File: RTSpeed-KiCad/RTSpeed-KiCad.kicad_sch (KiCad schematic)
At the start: 91 parts, among them J1 24V IN, J2 USB C Receptacle, J3 MOTOR, J4 -, J5 -, J6 -, J7 SWD-I^{2}C, J8 SENSORES HALL, Q1 DMG3402L, SW1 BOOT0, SW2 NRST, U1 STM32F411CEUx, U2 LM317L, U3 ADS7830, U4 LM317, Y1 25MHz, Y2 32.768kHz

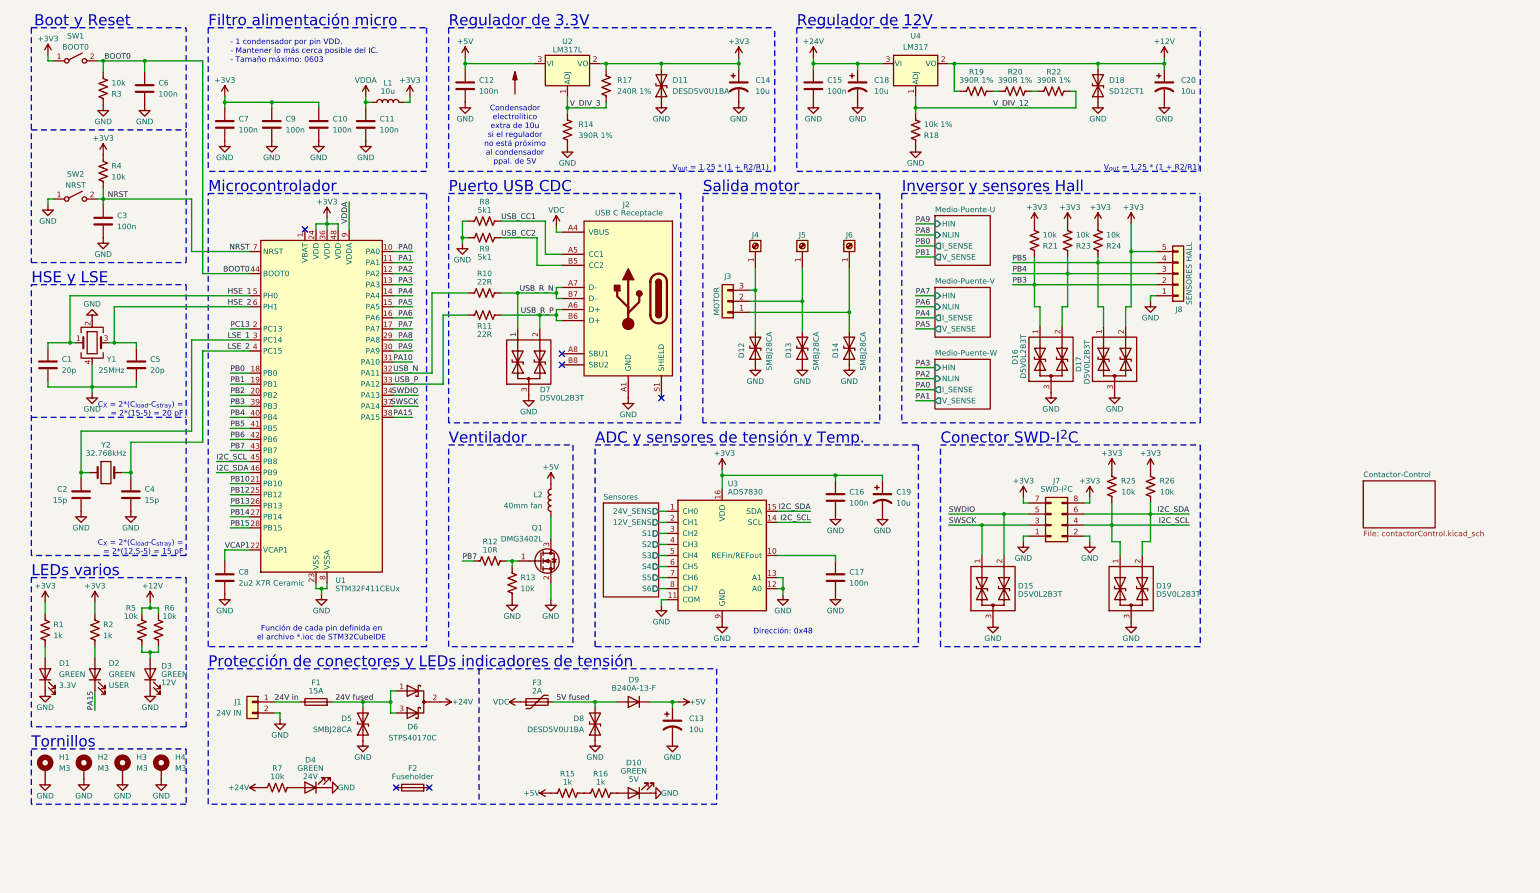
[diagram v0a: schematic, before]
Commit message: PCB redesign (not final)
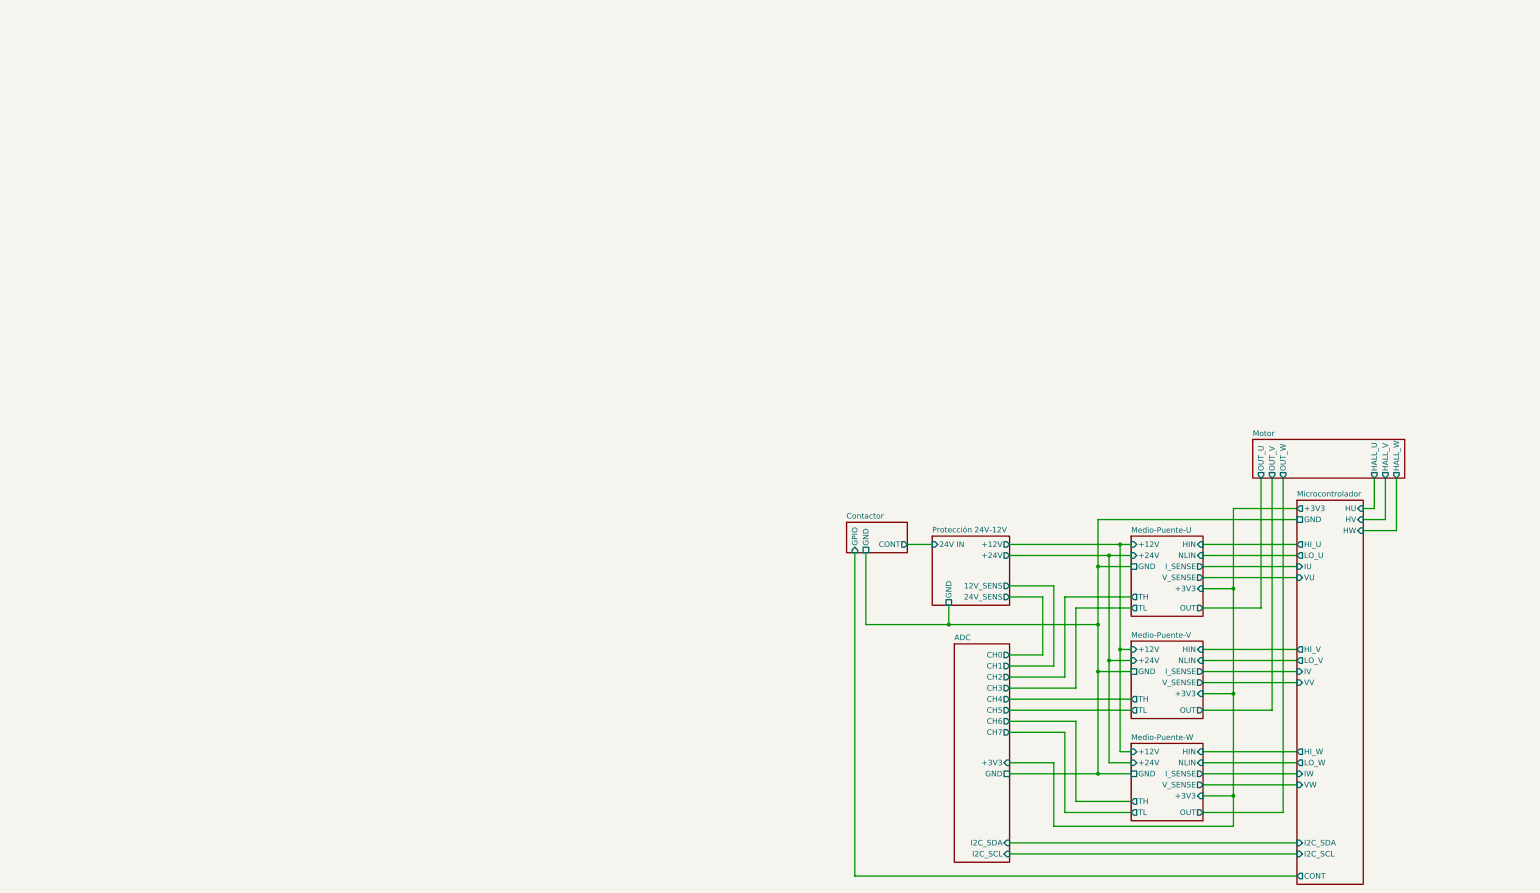
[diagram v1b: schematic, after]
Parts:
- removed C1, C5: 20p, Capacitor_SMD:C_0603_1608Metric, symbol Device:C
- removed C10, C11, C12, C15, C16, C17, C3, C6, C7, C9: 100n, Capacitor_SMD:C_0603_1608Metric, symbol Device:C
- removed C13, C14, C18, C19, C20: 10u, Capacitor_SMD:CP_Elec_4x5.4, symbol Device:C_Polarized_US
- removed C2, C4: 15p, Capacitor_SMD:C_0603_1608Metric, symbol Device:C
- removed C8: 2u2 X7R Ceramic, Capacitor_SMD:C_0603_1608Metric, symbol Device:C
- removed D1, D10, D2, D3, D4: GREEN, LED_SMD:LED_0805_2012Metric, symbol Device:LED
- removed D11, D8: DESD5V0U1BA, Diode_SMD:D_SOD-323_HandSoldering, symbol Device:D_TVS
- removed D12, D13, D14, D5: SMBJ28CA, Diode_SMD:D_SMB, symbol Device:D_TVS
- removed D15, D16, D17, D19, D7: D5V0L2B3T, Package_TO_SOT_SMD:SOT-523, symbol TFG-Brushless-ESC:Dual-TVS
- removed D18: SD12CT1, Diode_SMD:D_SOD-323_HandSoldering, symbol Device:D_TVS
- removed D6: STPS40170C, Package_TO_SOT_THT:TO-220-3_Vertical, symbol Device:D_Schottky_Dual_CommonCathode_AKA_Parallel
- removed D9: B240A-13-F, Diode_SMD:D_SMA, symbol Diode:1N4148W
- removed F1: 15A, TFG-Brushless-ESC:Fuseholder_Automotive, symbol Device:Fuse
- removed F2: Fuseholder, symbol Device:Fuse
- removed F3: 2A, Fuse:Fuse_1812_4532Metric, symbol Device:Polyfuse
- removed H1, H2, H3, H4: M3, MountingHole:MountingHole_3.2mm_M3_Pad_Via, symbol Mechanical:MountingHole_Pad
- removed J1: 24V IN, TFG-Brushless-ESC:Barrier_1x02, symbol Connector_Generic:Conn_01x02
- removed J2: USB C Receptacle, Connector_USB:USB_C_Receptacle_XKB_U262-16XN-4BVC11, symbol Connector:USB_C_Receptacle_USB2.0_16P
- removed J3: MOTOR, TFG-Brushless-ESC:Barrier_1x03, symbol Connector_Generic:Conn_01x03
- removed J4, J5, J6: -, MountingHole:MountingHole_2.5mm_Pad_TopBottom, symbol Connector:Screw_Terminal_01x01
- removed J7: SWD-I^{2}C, Connector_PinHeader_2.54mm:PinHeader_2x04_P2.54mm_Horizontal, symbol Connector_Generic:Conn_02x04_Odd_Even
- removed J8: SENSORES HALL, Connector_JST:JST_PH_S5B-PH-K_1x05_P2.00mm_Horizontal, symbol Connector_Generic:Conn_01x05
- removed L1: 10u, Inductor_SMD:L_0805_2012Metric, symbol Device:L
- removed L2: 40mm fan, Connector_JST:JST_PH_B2B-PH-K_1x02_P2.00mm_Vertical, symbol Device:L
- removed Q1: DMG3402L, Package_TO_SOT_SMD:SOT-23, symbol Transistor_FET:DMG3402L
- removed R1, R15, R16, R2: 1k, Resistor_SMD:R_0603_1608Metric, symbol Device:R_US
- removed R10, R11: 22R, Resistor_SMD:R_0603_1608Metric, symbol Device:R_US
- removed R12: 10R, Resistor_SMD:R_0805_2012Metric, symbol Device:R_US
- removed R13, R21, R23, R24, R25, R26, R3, R4, R5, R6, R7: 10k, Resistor_SMD:R_0603_1608Metric, symbol Device:R_US
- removed R14, R19, R20, R22: 390R 1%, Resistor_SMD:R_0603_1608Metric, symbol Device:R_US
- removed R17: 240R 1%, Resistor_SMD:R_0603_1608Metric, symbol Device:R_US
- removed R18: 10k 1%, Resistor_SMD:R_0603_1608Metric, symbol Device:R_US
- removed R8, R9: 5k1, Resistor_SMD:R_0603_1608Metric, symbol Device:R_US
- removed SW1: BOOT0, ESC-TFG-KiCad:SPDT, symbol Switch:SW_SPST
- removed SW2: NRST, ESC-TFG-KiCad:SPDT, symbol Switch:SW_SPST
- removed U1: STM32F411CEUx, Package_DFN_QFN:QFN-48-1EP_7x7mm_P0.5mm_EP5.6x5.6mm, symbol MCU_ST_STM32F4:STM32F411CEUx
- removed U2: LM317L, Package_TO_SOT_SMD:SOT-89-3, symbol Regulator_Linear:LM317L_SOT-89
- removed U3: ADS7830, Package_SO:TSSOP-16_4.4x5mm_P0.65mm, symbol Analog_DAC:ADS7830
- removed U4: LM317, Package_TO_SOT_THT:TO-220-3_Vertical, symbol Regulator_Linear:LM317_TO-220
- removed Y1: 25MHz, Oscillator:Oscillator_SMD_Abracon_ASE-4Pin_3.2x2.5mm, symbol Device:Crystal_GND24
- removed Y2: 32.768kHz, Crystal:Crystal_SMD_3215-2Pin_3.2x1.5mm, symbol Device:Crystal
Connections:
- no-connect marks 6 -> 0
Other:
- removed sheet Contactor-Control
- removed sheet Sensores
- added sheet ADC (ADC.kicad_sch)
- added sheet Contactor (Contactor.kicad_sch)
- added sheet Microcontrolador (Microcontrolador.kicad_sch)
- added sheet Motor (Motor.kicad_sch)
- added sheet Protección 24V-12V (Prot-24V-12V.kicad_sch)
- sheet Medio-Puente-U ports: added +12V, +24V, +3V3, GND, OUT, TH, TL; removed none
- sheet Medio-Puente-V ports: added +12V, +24V, +3V3, GND, OUT, TH, TL; removed none
- sheet Medio-Puente-W ports: added +12V, +24V, +3V3, GND, OUT, TH, TL; removed none
- note removed: "- 1 condensador por pin VDD. - Mantener lo más cerca posible del IC. - Tamaño máximo: 0603"
- note removed: "ADC y sensores de tensión y Temp."
- note removed: "Boot y Reset"
- note removed: "C_{X} = 2*(C_{load}-C_{stray}) = = 2*(12.5-5) = 15 pF"
- note removed: "C_{X} = 2*(C_{load}-C_{stray}) = = 2*(15-5) = 20 pF"
- note removed: "Condensador electrolítico extra de 10u si el regulador no está próximo al condensador ppal. de 5V"
- note removed: "Conector SWD-I^{2}C"
- note removed: "Dirección: 0x48"
- note removed: "Filtro alimentación micro"
- note removed: "Función de cada pin definida en el archivo *.ioc de STM32CubeIDE"
- note removed: "HSE y LSE"
- note removed: "Inversor y sensores Hall"
- note removed: "LEDs varios"
- note removed: "Microcontrolador"
- note removed: "Protección de conectores y LEDs indicadores de tensión"
- note removed: "Puerto USB CDC"
- note removed: "Regulador de 12V"
- note removed: "Regulador de 3.3V"
- note removed: "Salida motor"
- note removed: "Tornillos"
- note removed: "V_{out} = 1.25 * (1 + R2/R1)"
- note removed: "Ventilador"
